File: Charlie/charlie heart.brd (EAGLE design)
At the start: 46.7 x 57.7 mm, 32 parts, among them Q1 BSS84

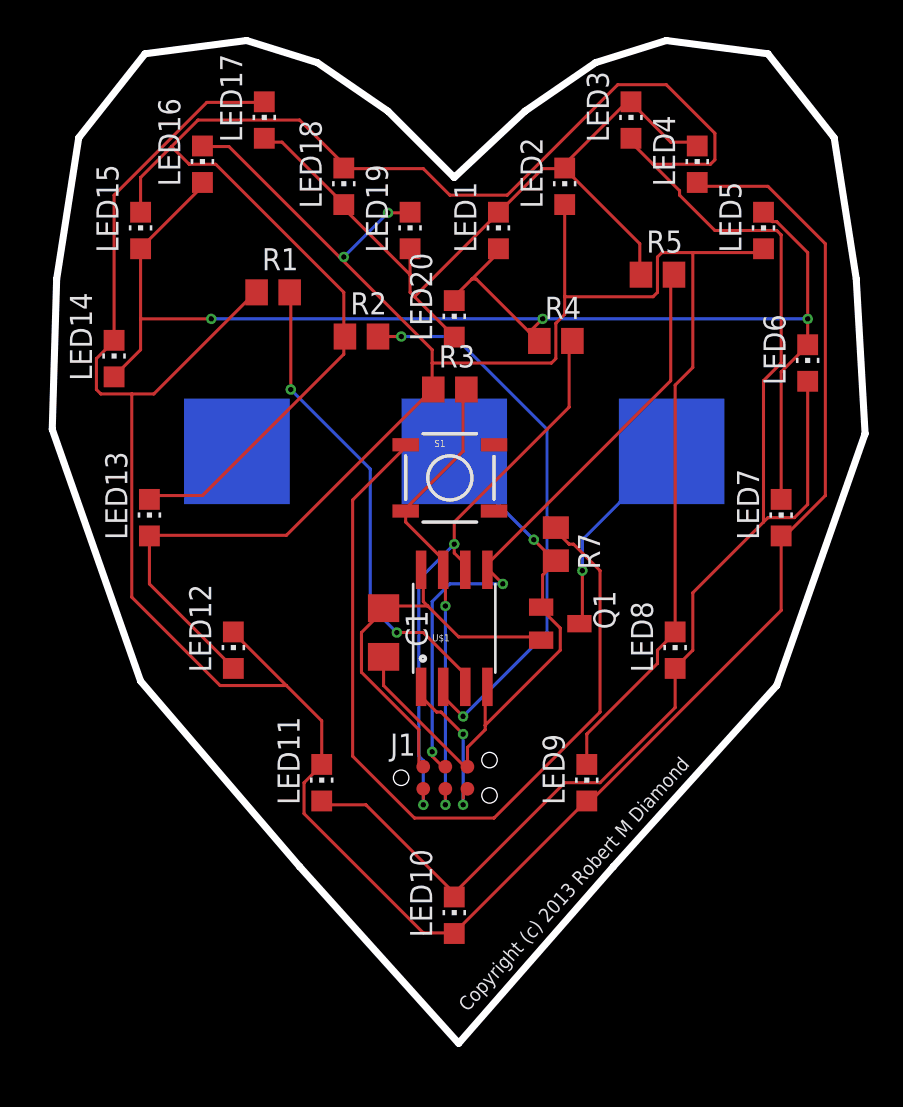
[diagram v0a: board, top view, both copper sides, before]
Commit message: update template
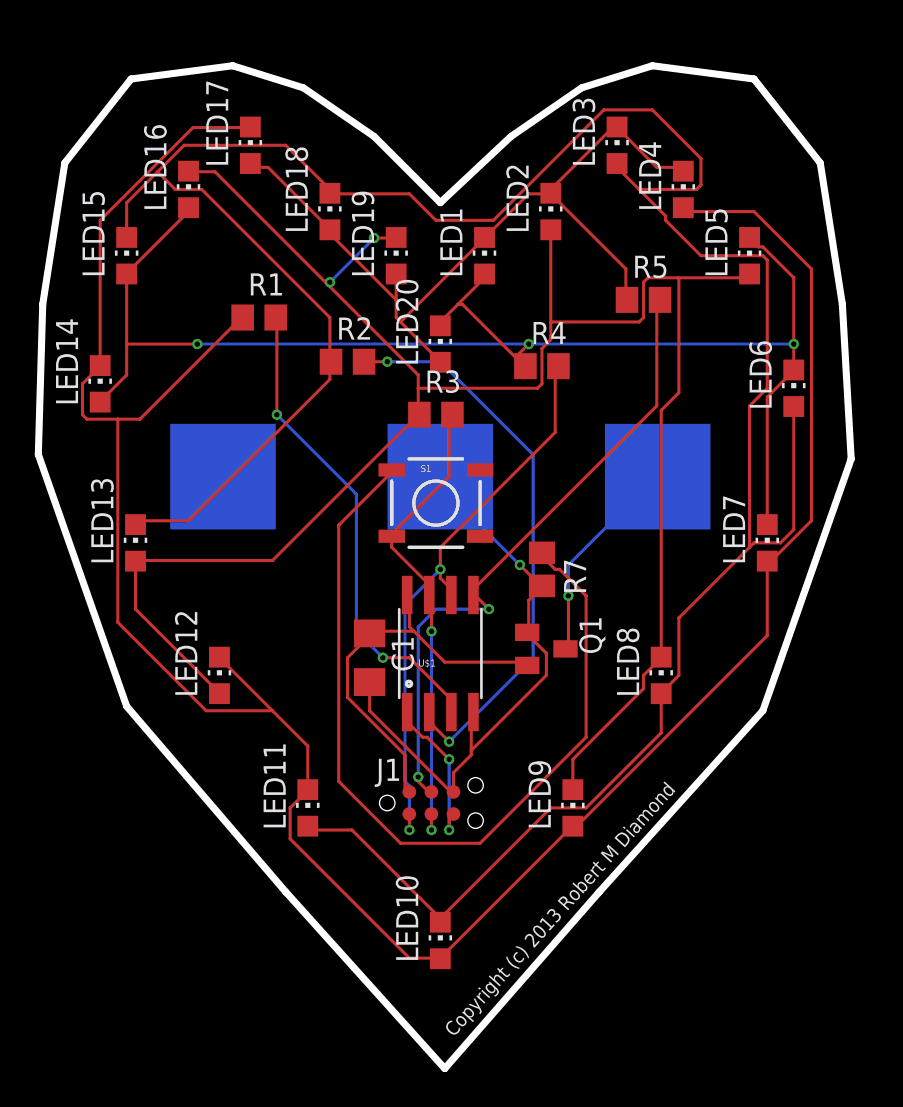
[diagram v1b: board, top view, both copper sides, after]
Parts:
- moved LED4 1.66 mm to (37.3, 50.6)
- moved LED6 1.66 mm to (43.6, 39.2)
- moved BAT1 1.66 mm to (23.3, 34.1)
- moved LED17 1.66 mm to (12.4, 53.2)
- moved LED20 1.66 mm to (23.3, 41.7)
- moved R2 1.66 mm to (18.0, 40.7)
- moved R3 1.66 mm to (23.1, 37.7)
- moved S1 1.66 mm to (23.1, 32.6)
- moved LED16 1.66 mm to (8.85, 50.6)
- moved R1 1.66 mm to (12.9, 43.3)
- moved LED7 1.66 mm to (42.1, 30.3)
- moved LED11 1.66 mm to (15.7, 15.1)
- moved LED9 1.66 mm to (30.9, 15.1)
- moved LED3 1.66 mm to (33.5, 53.2)
- moved LED10 1.66 mm to (23.3, 7.44)
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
